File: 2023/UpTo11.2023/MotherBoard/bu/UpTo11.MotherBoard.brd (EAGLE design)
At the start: 88 x 78 mm, 9 parts, among them X1 USB-A

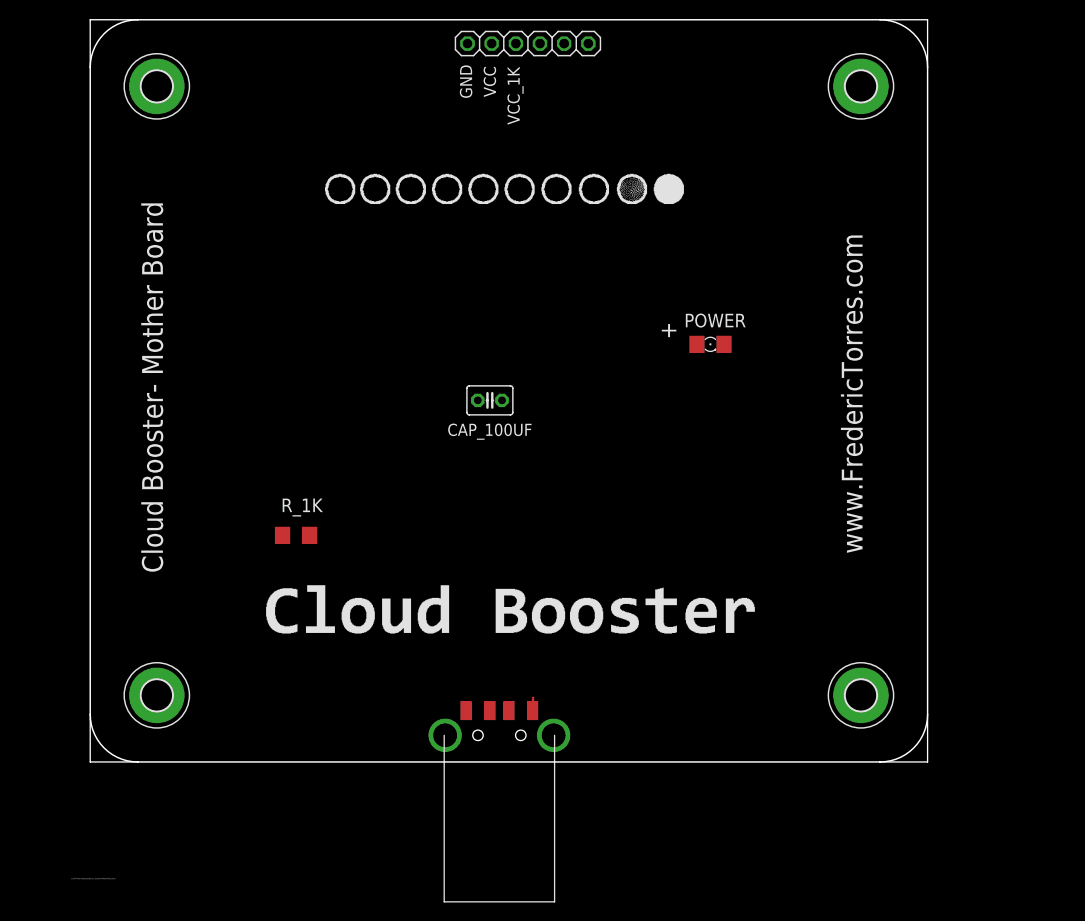
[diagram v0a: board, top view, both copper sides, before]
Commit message: Upto11 2023
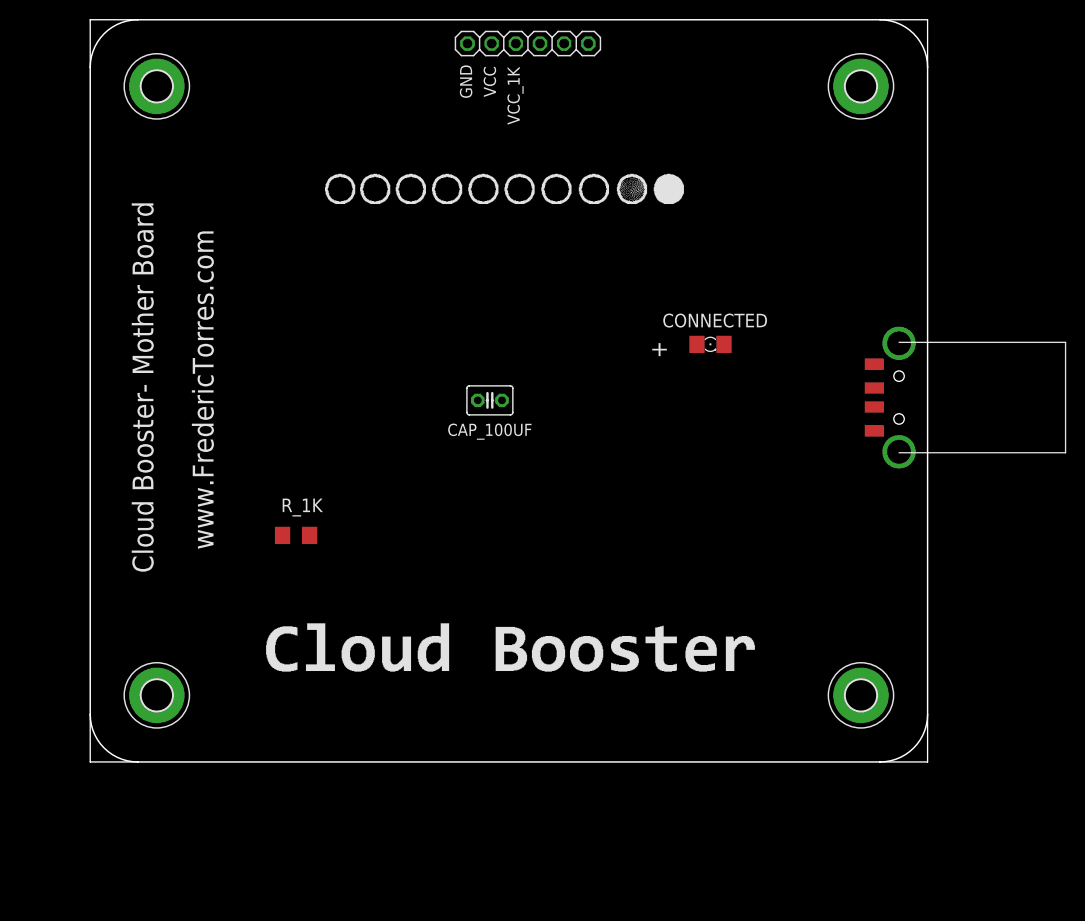
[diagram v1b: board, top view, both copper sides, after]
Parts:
- moved X1 55.0 mm to (87.0, 50.3), turned to 90 degrees
- renumbered POWER to CONNECTED
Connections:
- net VCC: no longer CONNECTED.A
- net VCC_1K: now also CONNECTED.A
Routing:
- net VCC: track 1.35 -> 0.00 mm
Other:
- board text added: "PCBv2 - 2023.08"
- board text removed: "C:/DVT/Fred.PCB/2023/UpTo11.2023/FrontPanel/Title1.bmp"
- board text removed: "MadeInTheUSB.net"
- board text removed: "PCBv1 - 2019.12"
- board text removed: "Up To 11 - MotherBoard"
- board text removed: "https://bit.ly/38Kq3UG"

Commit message: BNSK Booster v 2
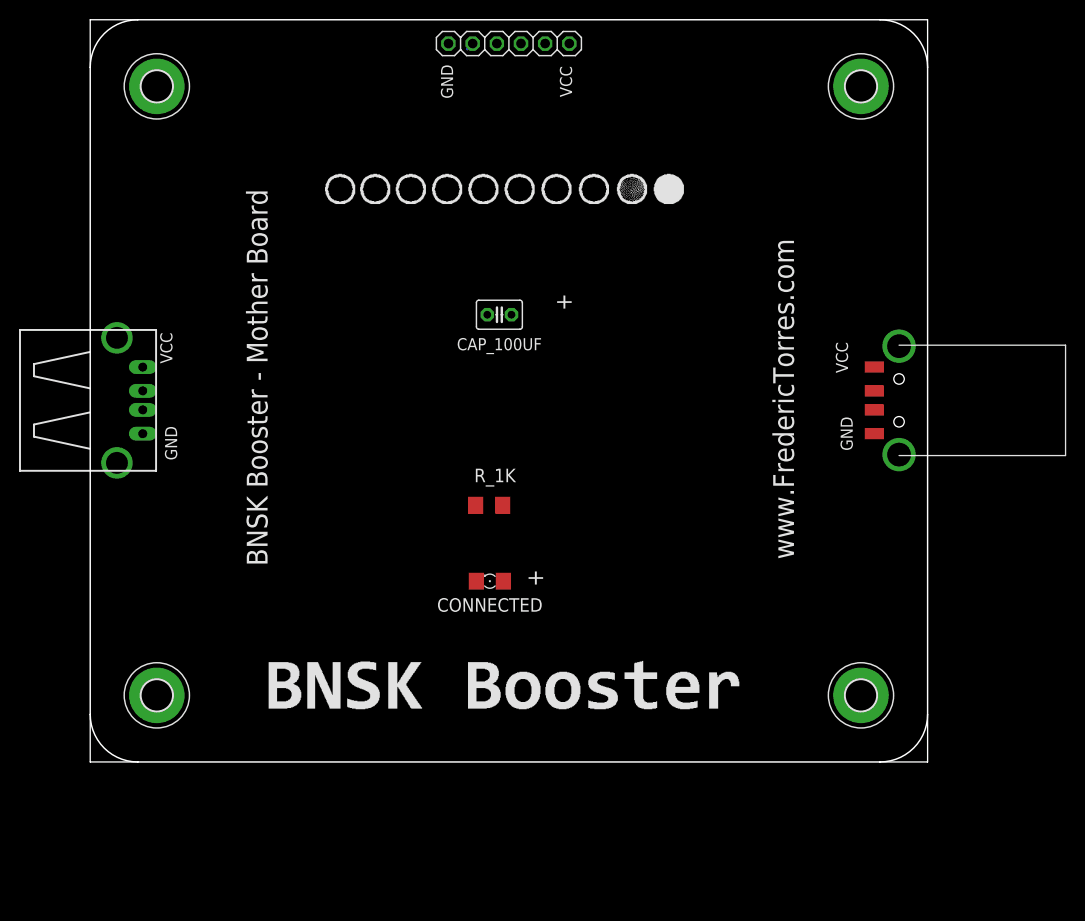
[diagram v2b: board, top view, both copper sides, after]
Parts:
- added CN1: (no value), microbuilder:USB_HOST-PTH
- moved CONNECTED 34.0 mm to (44.0, 31.0), turned to 180 degrees
- moved R_1K 20.5 mm to (43.9, 39.0)
- moved CAP_100UF 9.06 mm to (45.0, 59.0)
- moved FRONT_PANEL_INTERFACE 2.00 mm to (46.0, 87.5)
- moved X1 0.30 mm to (87.0, 50.0)
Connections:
- removed net VCC_1K: CAP_100UF.2, CONNECTED.A, FRONT_PANEL_INTERFACE.3, R_1K.1
- new net DMINUS: CN1.D+, X1.2
- new net DPLUS: CN1.D-, X1.3
- new net N$1: CONNECTED.A, R_1K.1
- net GND_EX: now also CN1.GND
- net VCC: now also CAP_100UF.2, CN1.VBUS, FRONT_PANEL_INTERFACE.6; no longer FRONT_PANEL_INTERFACE.2
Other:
- board text added: "BNSK Booster - Mother Board"
- board text removed: "Cloud Booster- Mother Board"
- board text removed: "VCC_1K"

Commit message: Fix usb female minus/plus
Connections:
- net DMINUS: now also CN1.D-; no longer CN1.D+
- net DPLUS: now also CN1.D+; no longer CN1.D-
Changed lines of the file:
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@@
 </signal>
 <signal name="DPLUS">
-<contactref element="CN1" pad="D-"/>
 <contactref element="X1" pad="3"/>
-<wire x1="7.52" y1="51" x2="84.4" y2="49" width="0" layer="19" extent="1-1"/>
+<contactref element="CN1" pad="D+"/>
+<wire x1="7.52" y1="49" x2="84.4" y2="49" width="0" layer="19" extent="1-1"/>
 </signal>
 <signal name="DMINUS">
-<contactref element="CN1" pad="D+"/>
 <contactref element="X1" pad="2"/>
-<wire x1="7.52" y1="49" x2="84.4" y2="51" width="0" layer="19" extent="1-1"/>
+<contactref element="CN1" pad="D-"/>
+<wire x1="7.52" y1="51" x2="84.4" y2="51" width="0" layer="19" extent="1-1"/>
 </signal>
 </signals>
